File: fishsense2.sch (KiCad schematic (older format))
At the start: 9 parts, among them J1 Conn_02x10_Odd_Even, Q1 Q_NMOS_GSD, SW1 SW_Reed

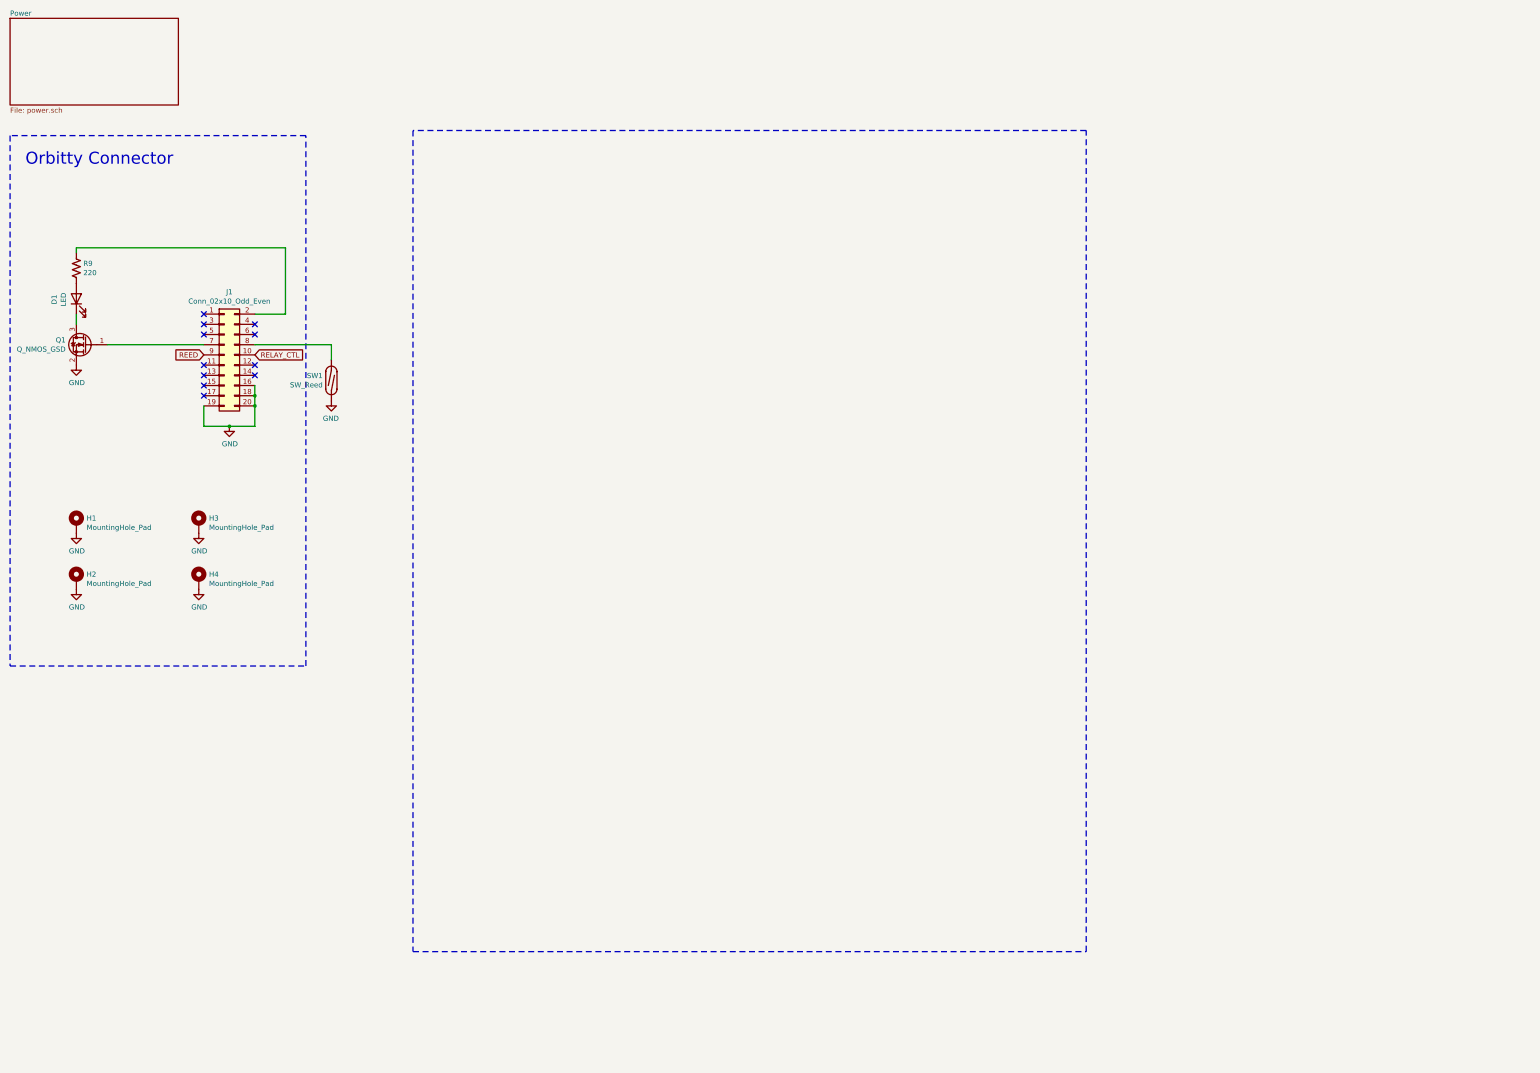
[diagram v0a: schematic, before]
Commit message: Many changes from first design review.
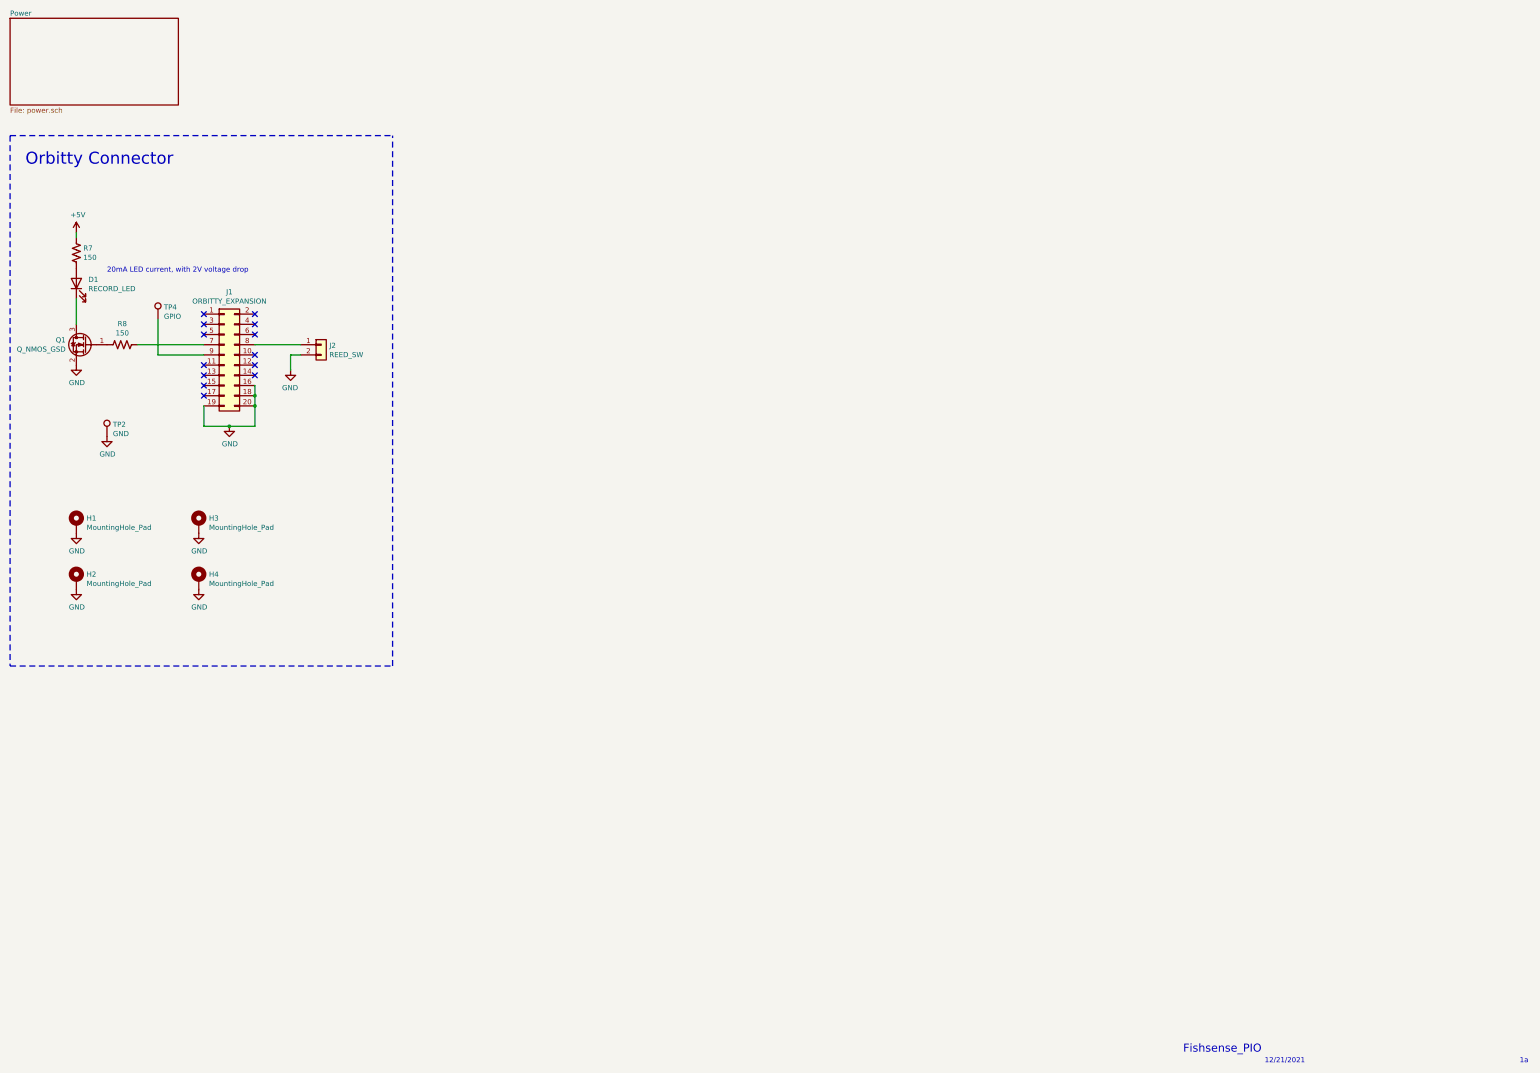
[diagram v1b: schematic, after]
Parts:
- removed R9: 220, Resistor_SMD:R_1206_3216Metric_Pad1.30x1.75mm_HandSolder, symbol Device:R_US
- removed SW1: SW_Reed, Connector_JST:JST_XH_S2B-XH-A_1x02_P2.50mm_Horizontal, symbol Switch:SW_Reed
- added J2: REED_SW, Connector_JST:JST_XH_S2B-XH-A_1x02_P2.50mm_Horizontal, symbol Connector_Generic:Conn_01x02
- added R7, R8: 150, Resistor_SMD:R_1206_3216Metric_Pad1.30x1.75mm_HandSolder, symbol Device:R_US
- added TP2: GND, TestPoint:TestPoint_Plated_Hole_D2.0mm, symbol Connector:TestPoint
- added TP4: GPIO, TestPoint:TestPoint_Plated_Hole_D2.0mm, symbol Connector:TestPoint
- D1: value LED -> RECORD_LED
- J1: value Conn_02x10_Odd_Even -> ORBITTY_EXPANSION; footprint Connector_PinHeader_2.54mm:PinHeader_2x10_P2.54mm_Vertical -> Connector_PinSocket_2.54mm:PinSocket_2x10_P2.54mm_Vertical
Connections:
- net GND: now also J2.2 (Pin_2), TP2.1
- net at D1.2 (A): now also R7.2
- net at J1.7 (Pin_7): now also R8.1; no longer Q1.1 (G)
- net at J1.8 (Pin_8): now also J2.1 (Pin_1)
- net REED: no longer names the net of J1.9 (Pin_9)
- net REED: now also TP4.1
- net RELAY_CTL: no longer names the net of J1.10 (Pin_10)
- new net: Q1.1 (G), R8.2
- new net +5V: R7.1
- no-connect marks 11 -> 13
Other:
- note added: "12/21/2021"
- note added: "1a"
- note added: "20mA LED current, with 2V voltage drop"
- note added: "Fishsense_PIO"
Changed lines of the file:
@@
 $EndDescr
-$Comp
-L Device:LED D1
-U 1 1 6166E725
-P 1350 3550
-F 0 "D1" H 1343 3767 50  0000 C CNN
-F 1 "LED" H 1343 3676 50  0000 C CNN
-F 2 "LED_THT:LED_D5.0mm_FlatTop" H 1350 3550 50  0001 C CNN
-F 3 "~" H 1350 3550 50  0001 C CNN
-	1    1350 3550
-	0    -1   -1   0
-$EndComp
 $Comp
 L Connector_Generic:Conn_02x10_Odd_Even J1
@@
 P 2800 4100
 F 0 "J1" H 2850 4717 50  0000 C CNN
-F 1 "Conn_02x10_Odd_Even" H 2850 4626 50  0000 C CNN
-F 2 "Connector_PinHeader_2.54mm:PinHeader_2x10_P2.54mm_Vertical" H 2800 4100 50  0001 C CNN
+F 1 "ORBITTY_EXPANSION" H 2850 4626 50  0000 C CNN
+F 2 "Connector_PinSocket_2.54mm:PinSocket_2x10_P2.54mm_Vertical" H 2800 4100 50  0001 C CNN
 F 3 "~" H 2800 4100 50  0001 C CNN
 	1    2800 4100
@@
 NoConn ~ 2600 4400
 NoConn ~ 2600 4500
-Text GLabel 2600 4100 0    50   Input ~ 0
-REED
-Text GLabel 3100 4100 2    50   Input ~ 0
-RELAY_CTL
-$Comp
-L Switch:SW_Reed SW1
-U 1 1 622296A5
-P 3850 4350
-F 0 "SW1" V 3896 4265 50  0000 R CNN
-F 1 "SW_Reed" V 3805 4265 50  0000 R CNN
-F 2 "Connector_JST:JST_XH_S2B-XH-A_1x02_P2.50mm_Horizontal" H 3850 4350 50  0001 C CNN
-F 3 "~" H 3850 4350 50  0001 C CNN
-	1    3850 4350
-	0    1    -1   0
-$EndComp
 $Comp
 L power:GND #PWR0128
 U 1 1 6222A48E
-P 3850 4550
-F 0 "#PWR0128" H 3850 4300 50  0001 C CNN
-F 1 "GND" H 3855 4377 50  0000 C CNN
-F 2 "" H 3850 4550 50  0001 C CNN
-F 3 "" H 3850 4550 50  0001 C CNN
-	1    3850 4550
+P 3450 4250
+F 0 "#PWR0128" H 3450 4000 50  0001 C CNN
+F 1 "GND" H 3455 4077 50  0000 C CNN
+F 2 "" H 3450 4250 50  0001 C CNN
+F 3 "" H 3450 4250 50  0001 C CNN
+	1    3450 4250
 	-1   0    0    -1
 $EndComp
-Wire Wire Line
-	3100 4000 3850 4000
-Wire Wire Line
-	3850 4000 3850 4150
-Wire Wire Line
-	2600 4000 1650 4000
 $Comp
 L power:GND #PWR0129
@@
 	1    0    0    -1
 $EndComp
-Wire Wire Line
-	1350 3700 1350 3800
-$Comp
-L Device:R_US R9
-U 1 1 61772274
-P 1350 3250
-F 0 "R9" H 1418 3296 50  0000 L CNN
-F 1 "220" H 1418 3205 50  0000 L CNN
-F 2 "Resistor_SMD:R_1206_3216Metric_Pad1.30x1.75mm_HandSolder" V 1390 3240 50  0001 C CNN
-F 3 "~" H 1350 3250 50  0001 C CNN
-	1    1350 3250
-	1    0    0    -1
-$EndComp
-Wire Wire Line
-	3100 3700 3400 3700
-Wire Wire Line
-	3400 3700 3400 3050
-Wire Wire Line
-	3400 3050 1350 3050
-Wire Wire Line
-	1350 3050 1350 3100
 Wire Notes Line width 20
 	700  1950 700  7150
 Wire Notes Line width 20
-	700  7150 3600 7150
-Wire Notes Line width 20
-	3600 7150 3600 1950
-Wire Notes Line width 20
-	3600 1950 700  1950
+	4450 7150 4450 1950
 Text Notes 850  2250 0    118  ~ 0
 Orbitty Connector
-Wire Notes Line width 20
-	4650 1900 4650 9950
-Wire Notes Line width 20
-	4650 9950 11250 9950
-Wire Notes Line width 20
-	11250 9950 11250 1900
-Wire Notes Line width 20
-	11250 1900 4650 1900
 $Comp
 L Device:Q_NMOS_GSD Q1
@@
 	-1   0    0    -1
 $EndComp
+Wire Notes Line width 20
+	700  7150 4450 7150
+Wire Notes Line width 20
+	700  1950 4450 1950
+NoConn ~ 3100 4100
+NoConn ~ 3100 3700
+$Comp
+L Device:LED D1
+U 1 1 61C3EDE1
+P 1350 3400
+F 0 "D1" V 1389 3282 50  0000 R CNN
+F 1 "RECORD_LED" V 1298 3282 50  0000 R CNN
+F 2 "LED_THT:LED_D5.0mm_FlatTop" H 1350 3400 50  0001 C CNN
+F 3 "~" H 1350 3400 50  0001 C CNN
+	1    1350 3400
+	0    -1   -1   0
+$EndComp
+$Comp
+L Device:R_US R7
+U 1 1 61C3EDE8
+P 1350 3100
+F 0 "R7" H 1418 3146 50  0000 L CNN
+F 1 "150" H 1418 3055 50  0000 L CNN
+F 2 "Resistor_SMD:R_1206_3216Metric_Pad1.30x1.75mm_HandSolder" V 1390 3090 50  0001 C CNN
+F 3 "~" H 1350 3100 50  0001 C CNN
+	1    1350 3100
+	1    0    0    -1
+$EndComp
+Wire Wire Line
+	1350 2900 1350 2950
+Wire Wire Line
+	1350 3550 1350 3800
+$Comp
+L power:+5V #PWR0106
+U 1 1 61C3F82C
+P 1350 2900
+F 0 "#PWR0106" H 1350 2750 50  0001 C CNN
+F 1 "+5V" H 1365 3073 50  0000 C CNN
+F 2 "" H 1350 2900 50  0001 C CNN
+F 3 "" H 1350 2900 50  0001 C CNN
+	1    1350 2900
+	1    0    0    -1
+$EndComp
+$Comp
+L Device:R_US R8
+U 1 1 61C42B26
+P 1800 4000
+F 0 "R8" V 1595 4000 50  0000 C CNN
+F 1 "150" V 1686 4000 50  0000 C CNN
+F 2 "Resistor_SMD:R_1206_3216Metric_Pad1.30x1.75mm_HandSolder" V 1840 3990 50  0001 C CNN
+F 3 "~" H 1800 4000 50  0001 C CNN
+	1    1800 4000
+	0    1    1    0
+$EndComp
+$Comp
+L power:GND #PWR0101
+U 1 1 61D8FB28
+P 1650 4900
+F 0 "#PWR0101" H 1650 4650 50  0001 C CNN
+F 1 "GND" H 1655 4727 50  0000 C CNN
+F 2 "" H 1650 4900 50  0001 C CNN
+F 3 "" H 1650 4900 50  0001 C CNN
+	1    1650 4900
+	1    0    0    -1
+$EndComp
+Wire Wire Line
+	3450 4250 3450 4100
+Wire Wire Line
+	3450 4100 3550 4100
+$Comp
+L Connector:TestPoint TP2
+U 1 1 61D8F5DF
+P 1650 4900
+F 0 "TP2" H 1708 5018 50  0000 L CNN
+F 1 "GND" H 1708 4927 50  0000 L CNN
+F 2 "TestPoint:TestPoint_Plated_Hole_D2.0mm" H 1850 4900 50  0001 C CNN
+F 3 "~" H 1850 4900 50  0001 C CNN
+	1    1650 4900
+	1    0    0    -1
+$EndComp
+$Comp
+L Connector_Generic:Conn_01x02 J2
+U 1 1 61D91AFB
+P 3750 4000
+F 0 "J2" H 3830 3992 50  0000 L CNN
+F 1 "REED_SW" H 3830 3901 50  0000 L CNN
+F 2 "Connector_JST:JST_XH_S2B-XH-A_1x02_P2.50mm_Horizontal" H 3750 4000 50  0001 C CNN
+F 3 "~" H 3750 4000 50  0001 C CNN
+	1    3750 4000
+	1    0    0    -1
+$EndComp
+Wire Wire Line
+	3550 4000 3100 4000
+Text Notes 1650 3300 0    50   ~ 0
+20mA LED current, with 2V voltage drop
+Text Notes 12200 10950 0    79   ~ 0
+Fishsense_PIO
+Text Notes 13000 11050 0    50   ~ 0
+12/21/2021
+Text Notes 15500 11050 0    50   ~ 0
+1a
+$Comp
+L Connector:TestPoint TP4
+U 1 1 61F33807
+P 2150 3750
+F 0 "TP4" H 2208 3868 50  0000 L CNN
+F 1 "GPIO" H 2208 3777 50  0000 L CNN
+F 2 "TestPoint:TestPoint_Plated_Hole_D2.0mm" H 2350 3750 50  0001 C CNN
+F 3 "~" H 2350 3750 50  0001 C CNN
+	1    2150 3750
+	1    0    0    -1
+$EndComp
+Wire Wire Line
+	1950 4000 2600 4000
+Wire Wire Line
+	2150 3750 2150 4100
+Wire Wire Line
+	2150 4100 2600 4100
 $EndSCHEMATC
